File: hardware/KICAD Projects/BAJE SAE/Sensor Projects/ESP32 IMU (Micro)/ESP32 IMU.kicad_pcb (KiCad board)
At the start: 2 copper layers, 30.5 x 73.3 mm, 8 parts, among them J1 Conn_01x02, J2 CAN to outer connector, J3 Conn_01x02, J4 Conn_01x02

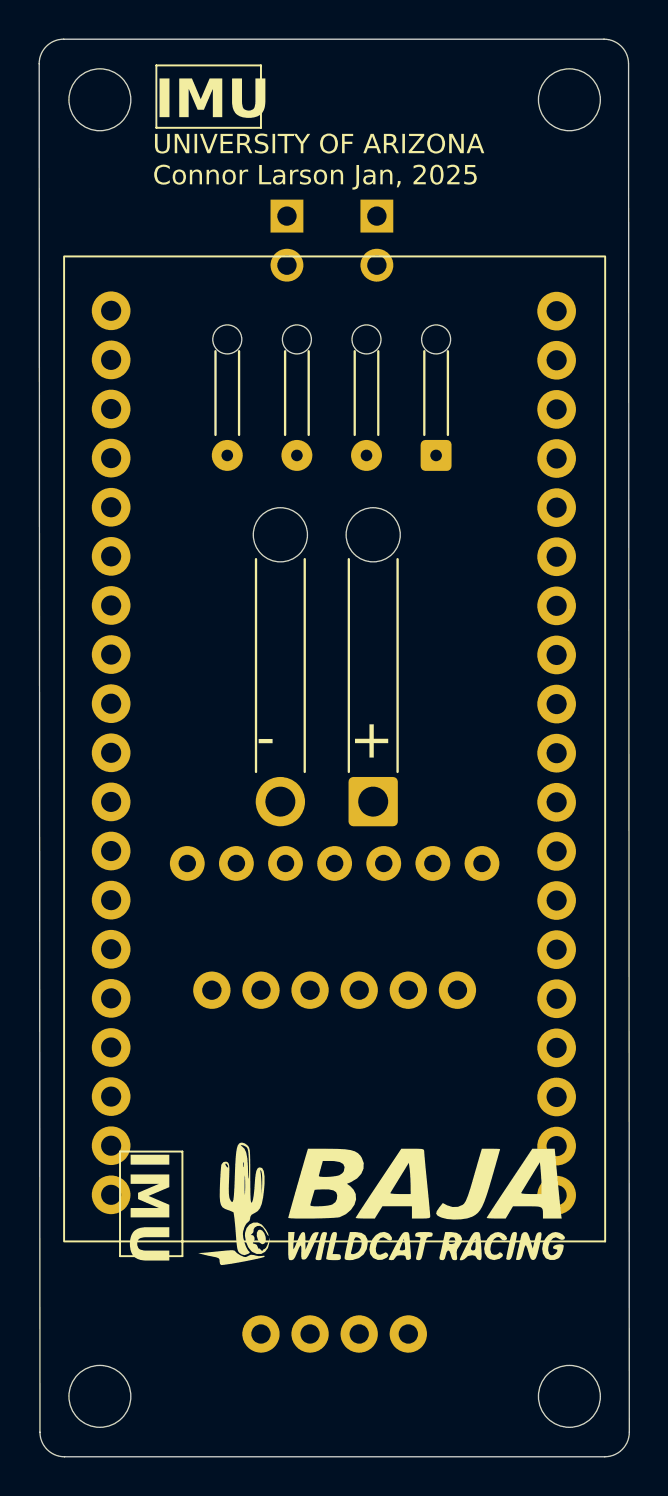
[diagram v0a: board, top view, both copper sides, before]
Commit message: finished imu, started others
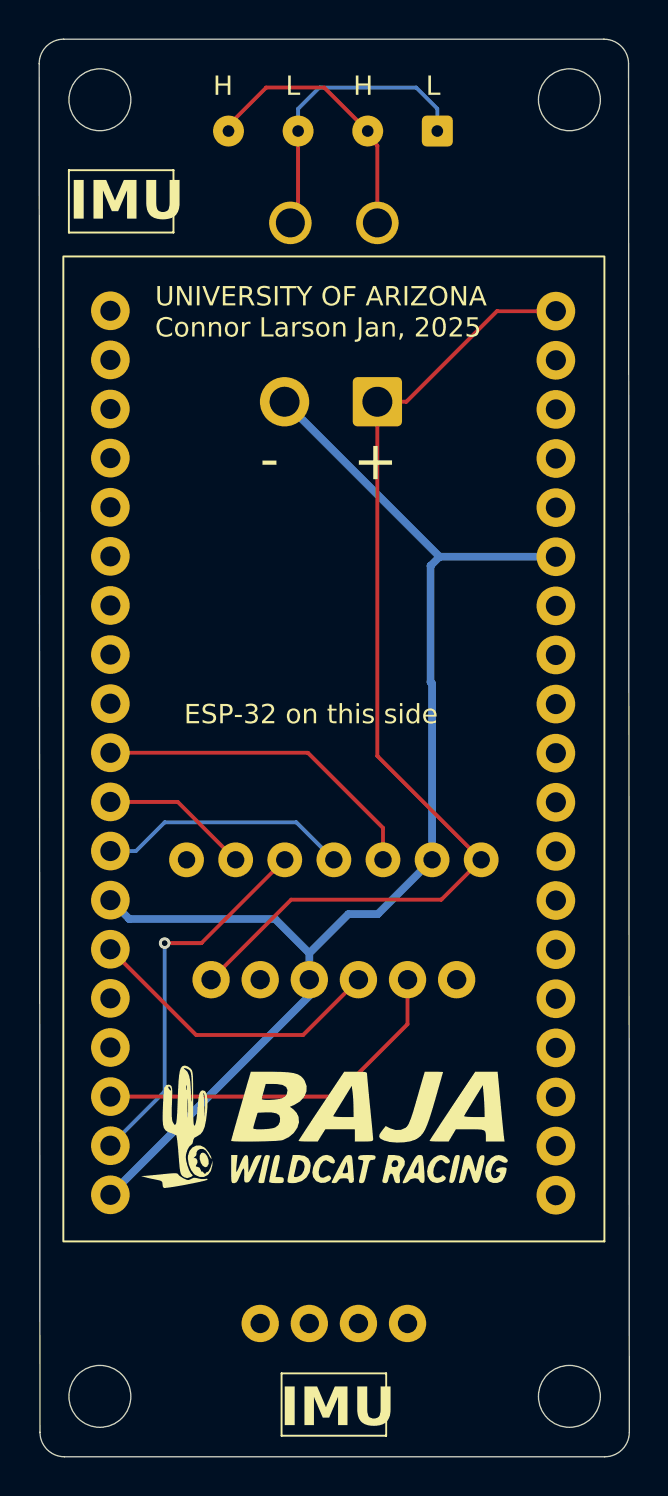
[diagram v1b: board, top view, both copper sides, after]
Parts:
- removed J3, J4: Conn_01x02, Connector_PinHeader_2.54mm:PinHeader_1x02_P2.54mm_Vertical
- J1: footprint Connector_Wire:SolderWire-0.75sqmm_1x02_P4.8mm_D1.25mm_OD2.3mm_Relief -> Connector_Wire:SolderWire-0.75sqmm_1x02_P4.8mm_D1.25mm_OD2.3mm
- J2: footprint Connector_Wire:SolderWire-0.1sqmm_1x04_P3.6mm_D0.4mm_OD1mm_Relief -> Connector_Wire:SolderWire-0.1sqmm_1x04_P3.6mm_D0.4mm_OD1mm
- moved J1 20.7 mm to (131.8, 76.5)
- moved J2 16.8 mm to (134.8, 62.5)
- moved CAN Bus (Facing UP) 8.09 mm to (127.1, 90.2)
- moved G*** 4.96 mm to (129.0, 114.0)
- moved UNIT_3 0.55 mm to (129.5, 115.3)
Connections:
- CAN Bus (Facing UP) pad 2: Net-(UNIT_1-IO18) -> SCK
- CAN Bus (Facing UP) pad 3: Net-(UNIT_1-IO23) -> SI
- CAN Bus (Facing UP) pad 4: Net-(UNIT_1-IO19) -> SO
- CAN Bus (Facing UP) pad 5: Net-(UNIT_1-IO5) -> CS
- J2 pad 1: /Green 1 -> Low
- J2 pad 2: /White 1 -> High
- J2 pad 3: /Green 2 -> Low
- J2 pad 4: /White 2 -> High
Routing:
- net GND: track 0.00 -> 69.8 mm
- net +5v: track 0.00 -> 53.6 mm
- net SI: track 0.00 -> 19.6 mm, vias 0 -> 1
- net SCL: track 0.00 -> 19.2 mm
- net CS: track 0.00 -> 17.4 mm
- net SDA: track 0.00 -> 15.8 mm
- net Low: track 0.00 -> 15.3 mm
- net High: track 0.00 -> 14.2 mm
- net SO: track 0.00 -> 13.0 mm
- net SCK: track 0.00 -> 7.72 mm
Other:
- board text added: "BNO on this side"
- board text added: "CAN BUS on this side"
- board text added: "ESP-32 on this side"
- board text added: "H"
- board text added: "L"
